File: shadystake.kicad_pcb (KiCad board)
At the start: 2 copper layers, 129.5 x 76.2 mm, 19 parts, among them J1 6P6C, J2 6P6C, J3 6P6C, J4 6P6C, J5 6P6C, J6 6P6C, J7 8P8C

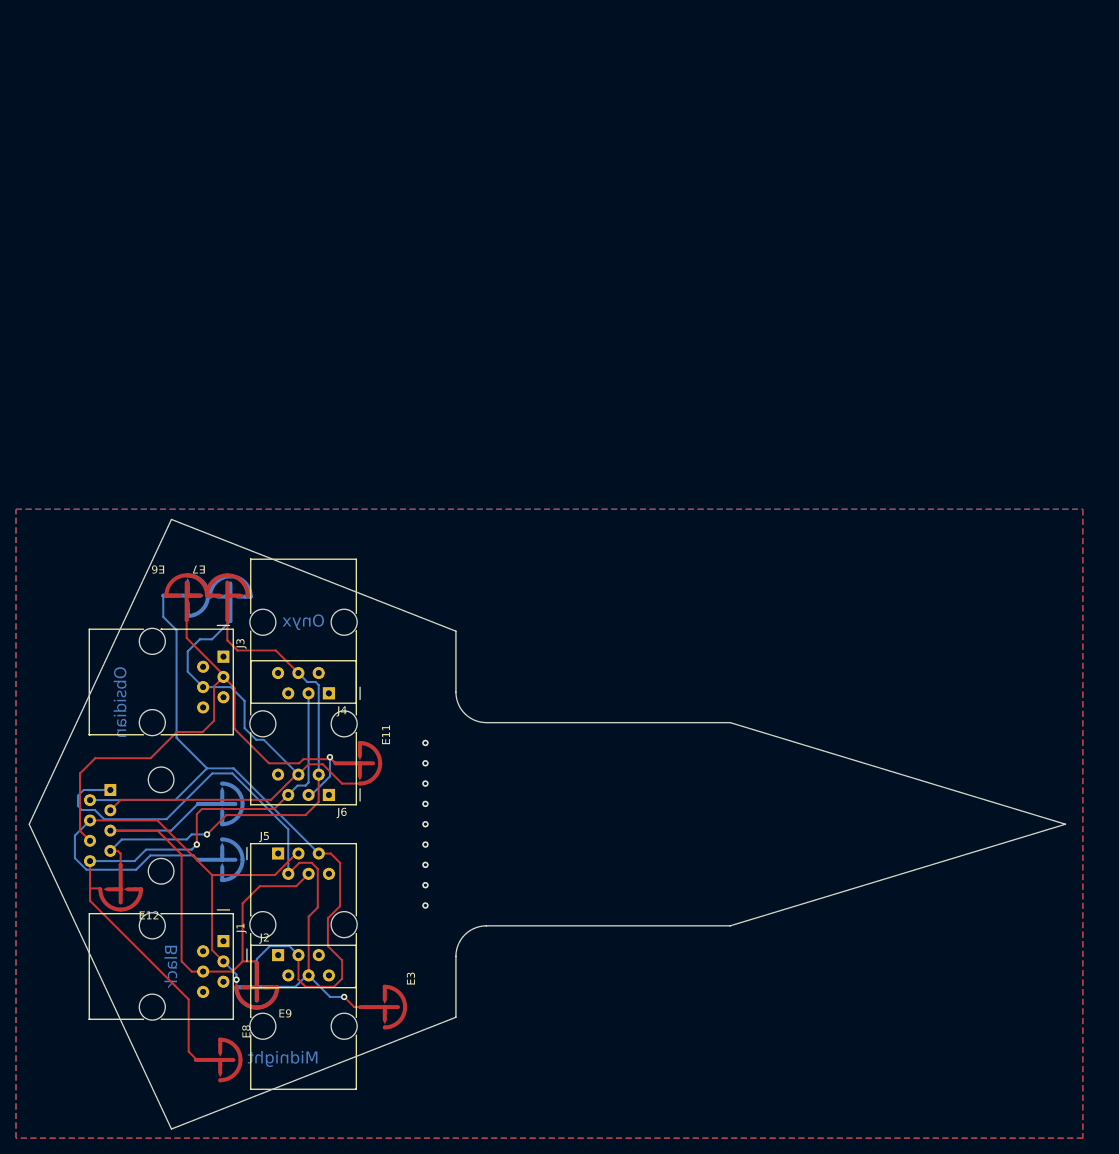
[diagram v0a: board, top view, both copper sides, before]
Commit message: Lay out design
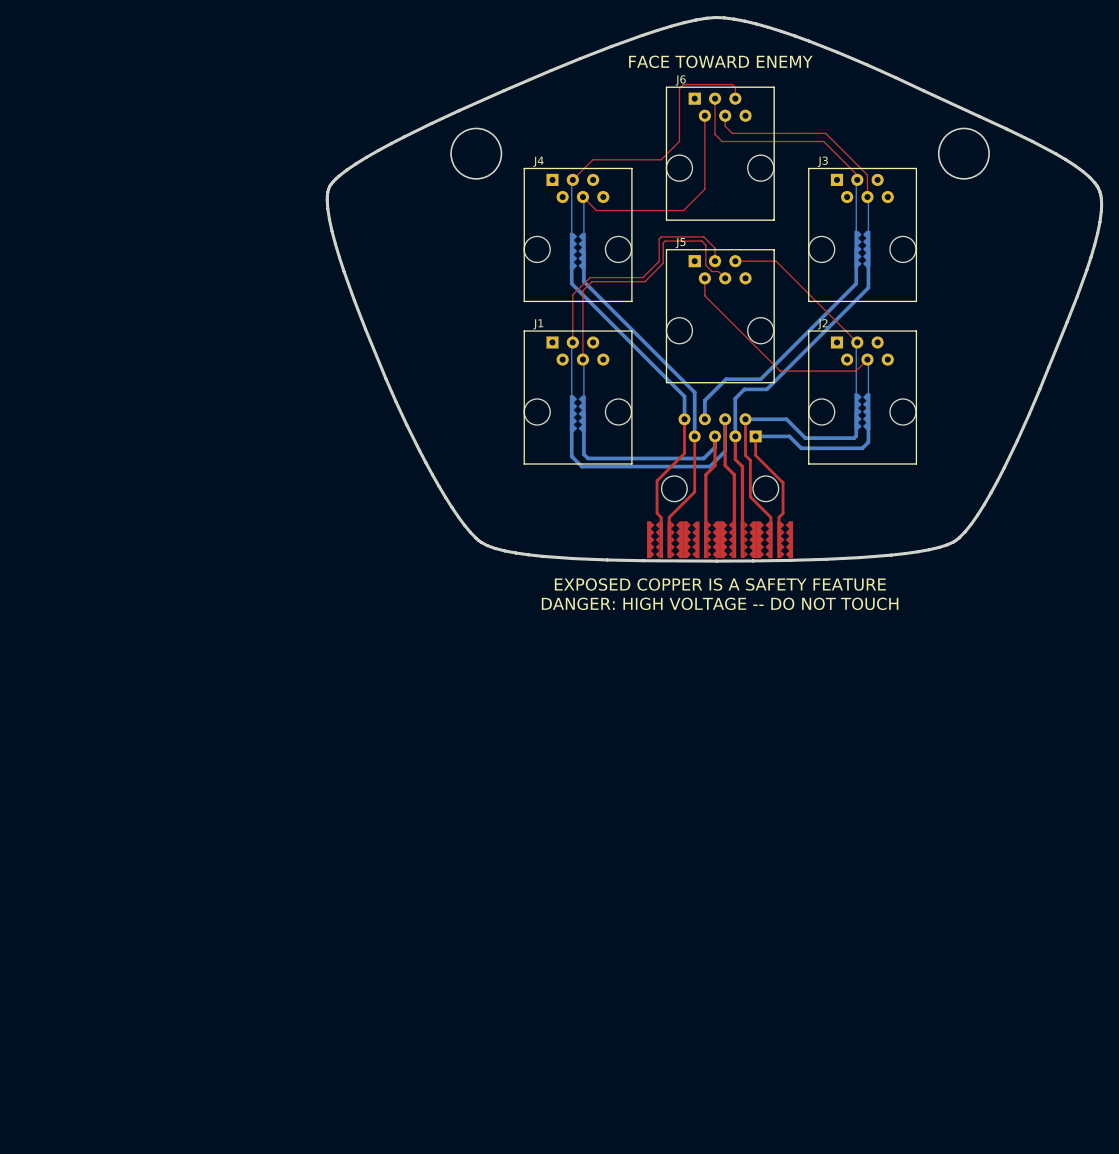
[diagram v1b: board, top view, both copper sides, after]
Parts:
- E1, E2, E4, E5: footprint Shadystake:Sparkgap_JLC -> Shadystake:Spark_Gap_Teeth; moved to F.Cu
- E10, E3, E6, E7, E8: footprint Shadystake:Sparkgap_JLC -> Shadystake:Spark_Gap_Teeth
- E11, E12, E9: footprint Shadystake:Sparkgap_JLC -> Shadystake:Spark_Gap_Teeth; moved to B.Cu
- J1, J2, J3, J4, J5, J6: footprint Connector_RJ:RJ12_Amphenol_54601 -> Shadystake:6P4C_Vert
- J7: footprint Connector_RJ:RJ45_Amphenol_54602-x08_Horizontal -> Shadystake:8P8C_Hor
- moved E10 104.4 mm to (152.4, 62.7)
- moved J2 103.8 mm to (149.2, 53.9)
- moved J6 98.5 mm to (131.4, 23.4), turned to 0 degrees
- moved E12 98.1 mm to (116.8, 42.7)
- moved J3 97.2 mm to (149.2, 33.6), turned to 0 degrees
- moved J7 91.9 mm to (139.1, 66.0), turned to 180 degrees
- moved J5 90.7 mm to (131.4, 43.7)
- moved E11 89.9 mm to (152.4, 42.4), turned to 180 degrees
- moved J1 85.6 mm to (113.7, 53.9), turned to 0 degrees
- moved E8 84.8 mm to (126.5, 78.7), turned to 0 degrees
- moved E9 82.2 mm to (116.8, 63.0)
- moved E3 76.9 mm to (142.7, 78.7), turned to 180 degrees
- moved E2 74.8 mm to (135.6, 78.7), turned to 0 degrees
- moved E4 72.5 mm to (140.2, 78.7), turned to 0 degrees
- moved J4 70.2 mm to (113.7, 33.6), turned to 0 degrees
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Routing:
- net /RING2: track 93.6 -> 62.7 mm
- net /RING1: track 67.5 -> 84.9 mm, vias 1 -> 0
- net /TIP4: track 62.3 -> 76.7 mm, vias 1 -> 0
- net /TIP1: track 63.5 -> 77.7 mm
- net /TIP3: track 64.9 -> 76.2 mm
- net /TIP2: track 74.1 -> 67.0 mm, vias 1 -> 0
- net /RING4: track 76.4 -> 83.2 mm, vias 1 -> 0
- net /RING3: track 71.7 -> 65.3 mm, vias 1 -> 0
- net Earth_Protective: vias 9 -> 0
- removed copper zone on B.Cu, net Earth_Protective
- removed copper zone on F.Cu, net Earth_Protective
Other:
- board size 129.5 x 76.2 mm -> 96.8 x 67.9 mm
- board text added: "EXPOSED COPPER IS A SAFETY FEATURE DANGER: HIGH VOLTAGE -- DO NOT TOUCH"
- board text added: "FACE TOWARD ENEMY"
- board text removed: "Black"
- board text removed: "Midnight"
- board text removed: "Obsidian"
- board text removed: "Onyx"
